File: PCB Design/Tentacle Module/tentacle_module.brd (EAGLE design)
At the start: 101.6 x 30.5 mm, 58 parts, among them IC1 5.0V, IC3 3.3V, T1 NTD5867NL, T2 NTD5867NL, T3 NTD5867NL, T4 NTD5867NL, U1 OKR-T/10-W12, X3 RJ45-8X, X4 RJ45-8X

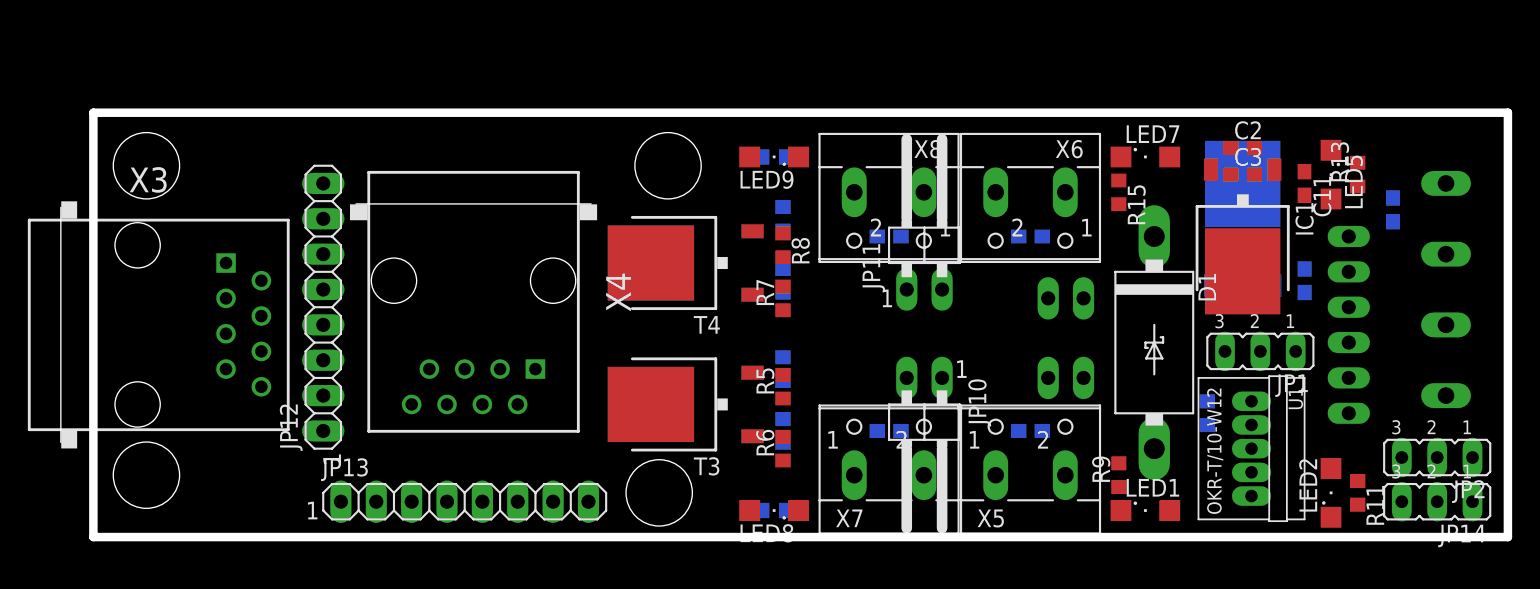
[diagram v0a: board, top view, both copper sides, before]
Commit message: Finished routing the Tentacle module board
Not changing it!
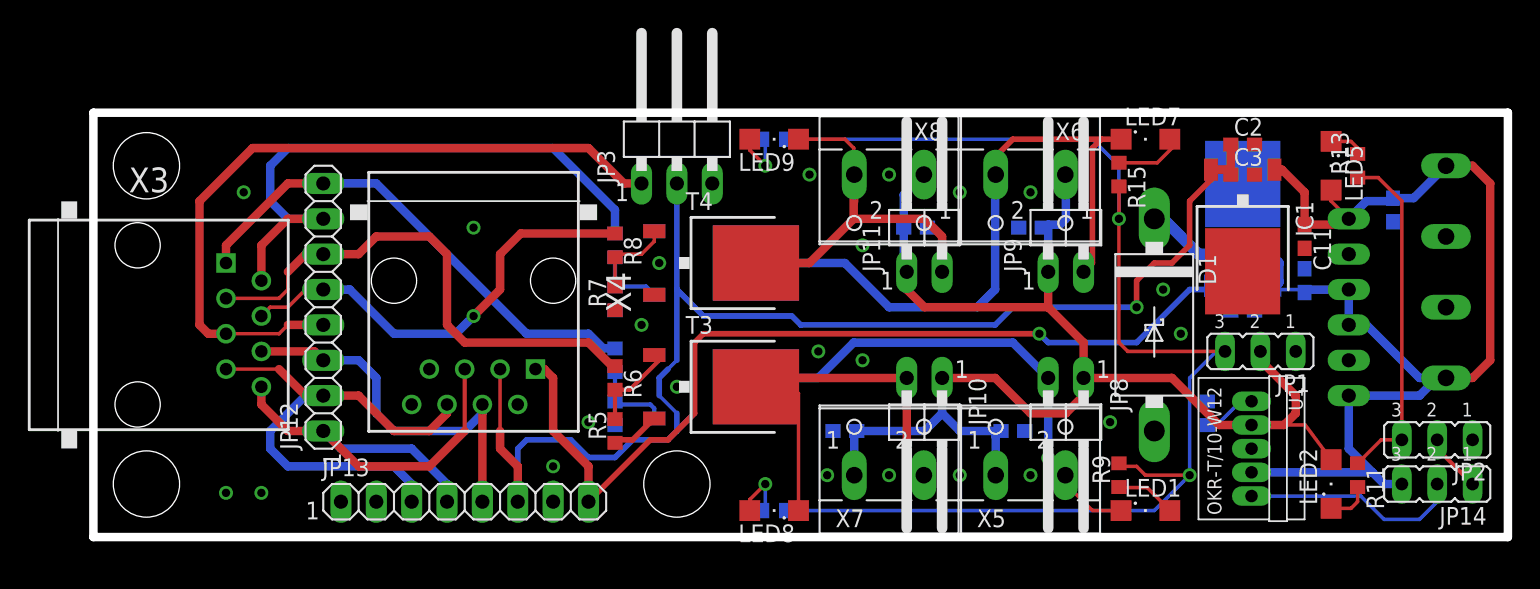
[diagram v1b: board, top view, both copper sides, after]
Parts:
- added JP3: (no value), CBLA_Test_bed_Library:1X03/90
- moved R3 13.1 mm to (37.5, 12.7)
- moved R6 13.1 mm to (37.5, 11.4), turned to 270 degrees
- moved R1 12.5 mm to (37.5, 8.89), turned to 90 degrees
- moved R5 12.5 mm to (37.5, 7.62)
- moved R4 12.2 mm to (37.5, 21.0)
- moved R2 12.1 mm to (37.5, 17.1)
- moved R7 12.1 mm to (37.5, 17.1)
- moved R8 12.1 mm to (37.5, 21.0)
- moved C11 3.81 mm to (87.0, 21.6)
- moved C8 3.17 mm to (54.0, 7.62)
- moved T1 2.84 mm to (45.1, 10.8), turned to 90 degrees
- moved T3 2.84 mm to (45.1, 10.8), turned to 270 degrees
- moved T2 2.54 mm to (45.1, 19.7), turned to 90 degrees
- moved T4 2.54 mm to (45.1, 19.7), turned to 270 degrees
- moved C9 2.01 mm to (59.1, 22.2)
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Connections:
- removed net +3V3: C4.1, C5.1, IC3.3
- net +3.3V: now also C4.1, C5.1, IC3.3
- net +5V: now also JP3.2
- net GND: now also D1.A, JP3.3, X1.2
- net IR1: now also JP3.1
- net PWR_LED_GND: no longer D1.A, X1.2
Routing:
- net +5V: track 0.00 -> 99.9 mm, vias 0 -> 1
- net +5V_HI-PWR: track 0.00 -> 99.8 mm
- net +12V: track 0.00 -> 94.0 mm
- net TEST_LED_V+: track 0.00 -> 93.4 mm, vias 0 -> 2
- net +3.3V: track 0.00 -> 69.9 mm, vias 0 -> 1
- net IR1: track 0.00 -> 52.7 mm
- net SMA2_OUT-: track 0.00 -> 48.4 mm
- net PWM2: track 0.00 -> 43.5 mm
- net SCL: track 0.00 -> 37.5 mm
- net PWM3: track 0.00 -> 37.4 mm
- net SMA1_OUT-: track 0.00 -> 36.5 mm, vias 0 -> 1
- net PWM1: track 0.00 -> 36.0 mm
- net SDA: track 0.00 -> 35.0 mm
- net PWM4: track 0.00 -> 32.0 mm, vias 0 -> 1
- net SMA4_OUT-: track 0.00 -> 29.1 mm
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- added copper zone on layer 1, net GND
- added copper zone on layer 16, net GND
